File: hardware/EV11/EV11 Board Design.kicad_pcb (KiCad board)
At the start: 4 copper layers, 68.4 x 89.4 mm, 103 parts, among them J1 Conn_01x02_Socket, J10 Conn_01x08_Socket, J11 Conn_01x06_Female, J13 Conn_01x04_Female, J4 AudioPlug4, J5 Conn_01x02_Socket, J7 Conn_01x04_Female, J9 USB_C_Receptacle, SW4 SW_Push, SW5 SW_Push, U1 STM32F405RGTx, U11 ESP32-S3-WROOM-1-N8R2, U13 BM14B(0.8)-24DS-0.4V(53), U2 BQ21040DBVR, U3 CH340C, U4 USBLC6-2P6, U5 STM32F030C8Tx, U6 WM8960CGEFL/RV, U7 TPS63060, Y1 Crystal_GND24

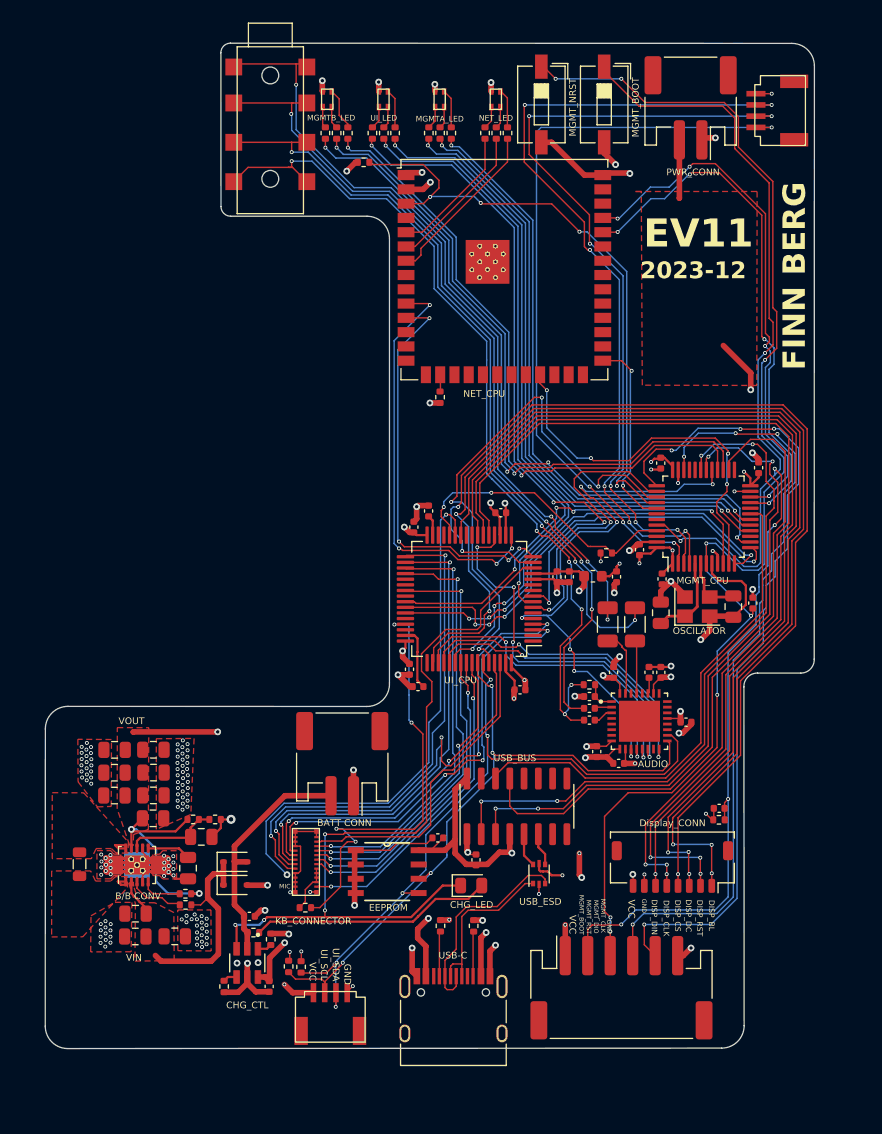
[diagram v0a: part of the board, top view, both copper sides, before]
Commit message: Added another test point to EV10.1 for BCLK. EV11 WIP
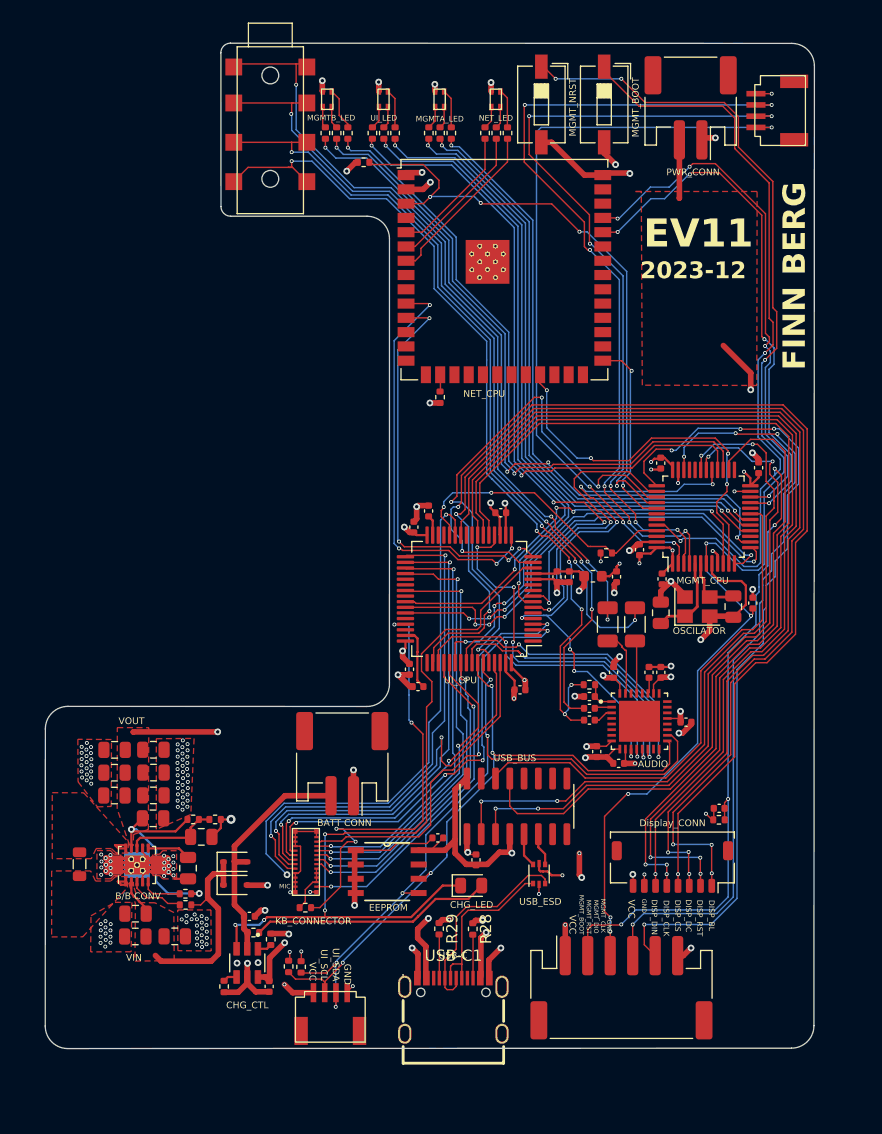
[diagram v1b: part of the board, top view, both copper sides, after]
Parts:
- removed J9: USB_C_Receptacle, Connector_USB:USB_C_Receptacle_HRO_TYPE-C-31-M-12
- removed R2, R3: 5k1, Resistor_SMD:R_0402_1005Metric
- added R28: 5k1, Resistor_SMD:R_0402_1005Metric, F.Cu at (152.0, 134.8)
- added R29: 5k1, Resistor_SMD:R_0402_1005Metric, F.Cu at (149.0, 134.8)
- added USB-C1: TYPE-C-31-M-12, footprint:USB-C_SMD-TYPE-C-31-M-12, F.Cu at (150.3, 141.6)
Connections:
- U1 pad 52: /I2S_ADCDAT -> /KB_ROW7
- U1 pad 53: /I2S_DACDAT -> /KB_COL5
- U1 pad 56: /KB_ROW7 -> /I2S_ADCDAT
- U1 pad 57: /KB_COL5 -> /I2S_DACDAT
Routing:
- net Net-(J9-CC1): track 4.17 -> 0.00 mm
- net Net-(J9-CC2): track 3.99 -> 0.00 mm
- net Net-(USB-C1-CC1): track 0.00 -> 3.89 mm
- net Net-(USB-C1-CC2): track 0.00 -> 3.87 mm
- net /I2S_ADCDAT: track 28.4 -> 26.6 mm
- net GND: track 552.7 -> 554.3 mm
- net /I2S_DACDAT: track 26.8 -> 25.5 mm
- net /MGMT_NRST: track 117.8 -> 116.6 mm
- net /DISP_CS: track 94.1 -> 94.7 mm
- net /KB_COL5: track 26.6 -> 27.2 mm
- net /USB_TX1_MGMT: track 61.5 -> 62.0 mm
- net /USB_RX1_MGMT: track 59.6 -> 60.1 mm
- net /USB_DTR: track 59.0 -> 59.5 mm
- net /DISP_RSTR: track 85.8 -> 86.3 mm
- net /USB_RTS: track 44.5 -> 45.1 mm
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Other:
- outline, holes or cut-outs redrawn
